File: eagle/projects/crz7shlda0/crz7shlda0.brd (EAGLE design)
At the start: 51.2 x 50 mm, 30 parts, among them J3 HDR-2X8, J5 HDR-2X8, Q1 BSS138, Q5 BSS138, Q6 BSS138, T1 MMBT3904

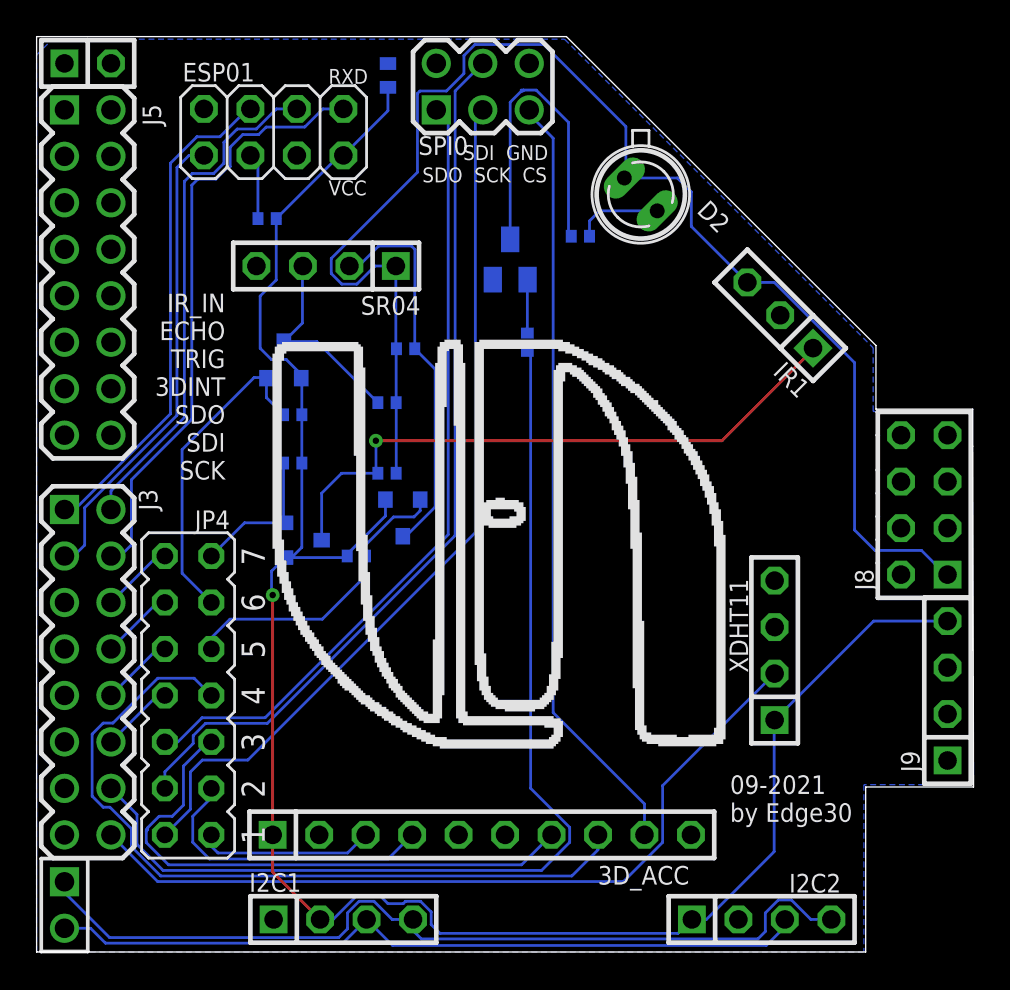
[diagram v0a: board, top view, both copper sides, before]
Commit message: cmod7shld0, crz7shlda0 production
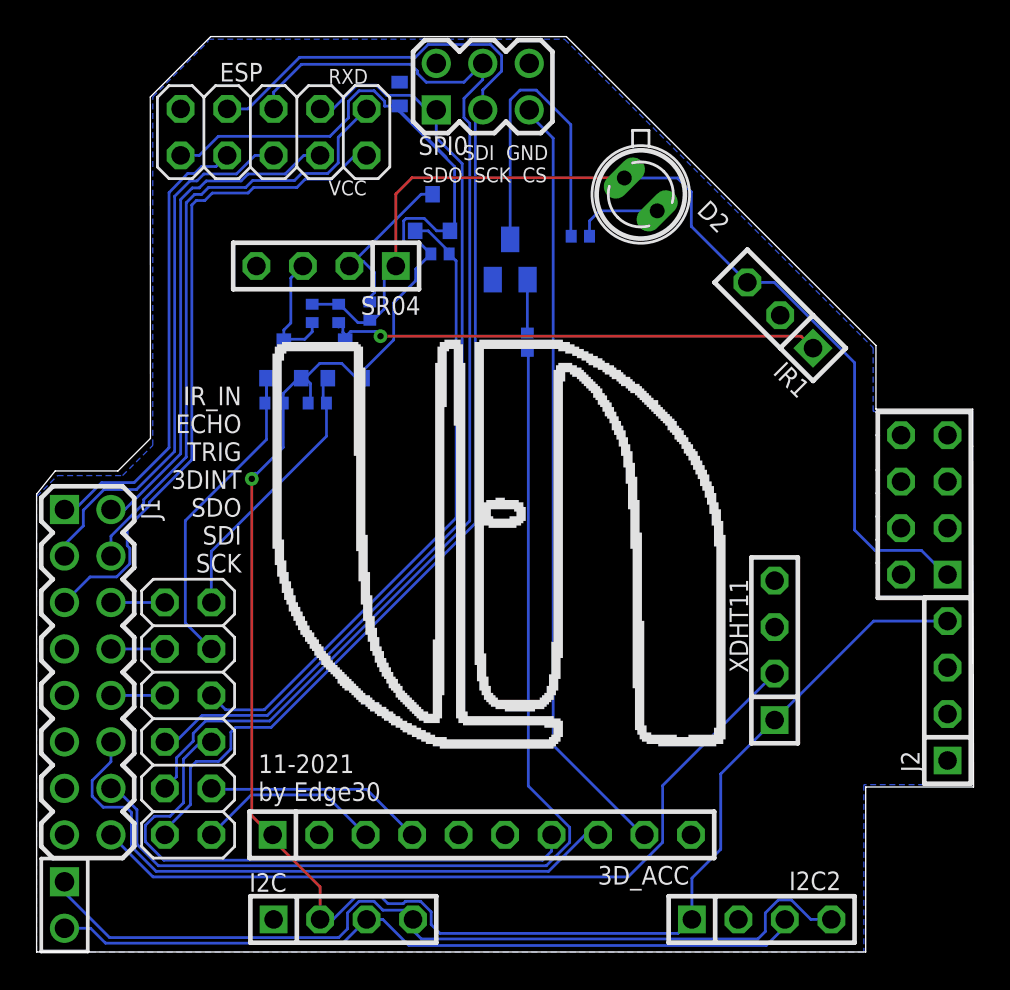
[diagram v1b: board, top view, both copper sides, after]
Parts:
- removed ESP01: (no value), pinhead:2X04
- removed J5: HDR-2X8, Mechanical:HDR-2X8
- removed J5G: (no value), pinhead2:1X02
- removed R19: 10k, rcl:R0402
- added ESP: (no value), pinhead:2X05
- I2C: value (none) -> I2C
- I2C2: value (none) -> I2Crev
- JP4: device jumper:JP7Q -> pinhead:2X06
- moved R17 17.1 mm to (22.0, 38.2)
- moved Q6 16.8 mm to (21.6, 40.4), turned to 0 degrees
- moved Q1 10.1 mm to (16.9, 32.4), turned to 0 degrees
- moved R14 9.13 mm to (16.5, 34.9), turned to 90 degrees
- moved R13 6.36 mm to (15.1, 34.9), turned to 90 degrees
- moved R15 3.54 mm to (15.3, 30.0), turned to 180 degrees
- moved R5 2.84 mm to (18.2, 35.0), turned to 270 degrees
- moved JP4 1.27 mm to (8.28, 12.8)
- moved C3 1.20 mm to (19.8, 46.9)
- moved R16 1.20 mm to (13.0, 30.0)
- renumbered I2C1 to I2C, J3 to J1, J9 to J2
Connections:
- removed net 3DIRQ: 3D_ACC.8, JP4.7
- removed net GPO0: ESP01.6, J1.2
- removed net GPO2: ESP01.4, J1.1
- removed net KCHIP_EN: ESP01.3, R19.2
- removed net URXD: ESP01.8, J1.4
- removed net UTXD: ESP01.1, J1.3
- new net CS2: ESP.10, J1.4
- new net EN_ESP: ESP.7, J1.2
- new net GPIO3: ESP.3, J1.1
- new net GPIO8: ESP.9, J1.5
- new net GPIO9: ESP.5, J1.3
- net 3D_INT: now also 3D_ACC.8; no longer JP4.8
- net ECHOIN: now also JP4.10; no longer JP4.12
- net ECHO_: now also JP4.9; no longer JP4.11
- net IRIN: now also JP4.12; no longer JP4.14
- net IR_OUT_: now also JP4.11; no longer JP4.13
- net K3V: now also ESP.1; no longer ESP01.7, R19.1
- net KGND: now also ESP.2; no longer ESP01.2, J5G.1, J5G.2
- net SCK: now also ESP.4
- net SDI: now also ESP.6
- net SDO: now also ESP.8
- net TRIGOUT: now also JP4.8; no longer JP4.10
- net TRIG_: now also JP4.7; no longer JP4.9
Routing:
- net 3DIRQ: track 43.0 -> 0.00 mm
- net GPIO8: track 0.00 -> 36.2 mm
- net CS2: track 0.00 -> 33.8 mm
- net URXD: track 33.0 -> 0.00 mm
- net 3D_INT: track 4.00 -> 34.7 mm
- net GPIO9: track 0.00 -> 29.5 mm
- net GPO0: track 28.1 -> 0.00 mm
- net EN_ESP: track 0.00 -> 27.6 mm
- net GPO2: track 27.3 -> 0.00 mm
- net UTXD: track 25.8 -> 0.00 mm
- net GPIO3: track 0.00 -> 25.1 mm
- net K5V: track 78.4 -> 57.4 mm
- net SCK: track 48.3 -> 68.8 mm
- net K3V: track 107.3 -> 126.8 mm
- net TRIG_: track 17.3 -> 35.4 mm
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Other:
- outline, holes or cut-outs redrawn
- board text added: "11-2021 by Edge30"
- board text removed: "09-2021 by Edge30"

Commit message: just push latest hanging changes to repo
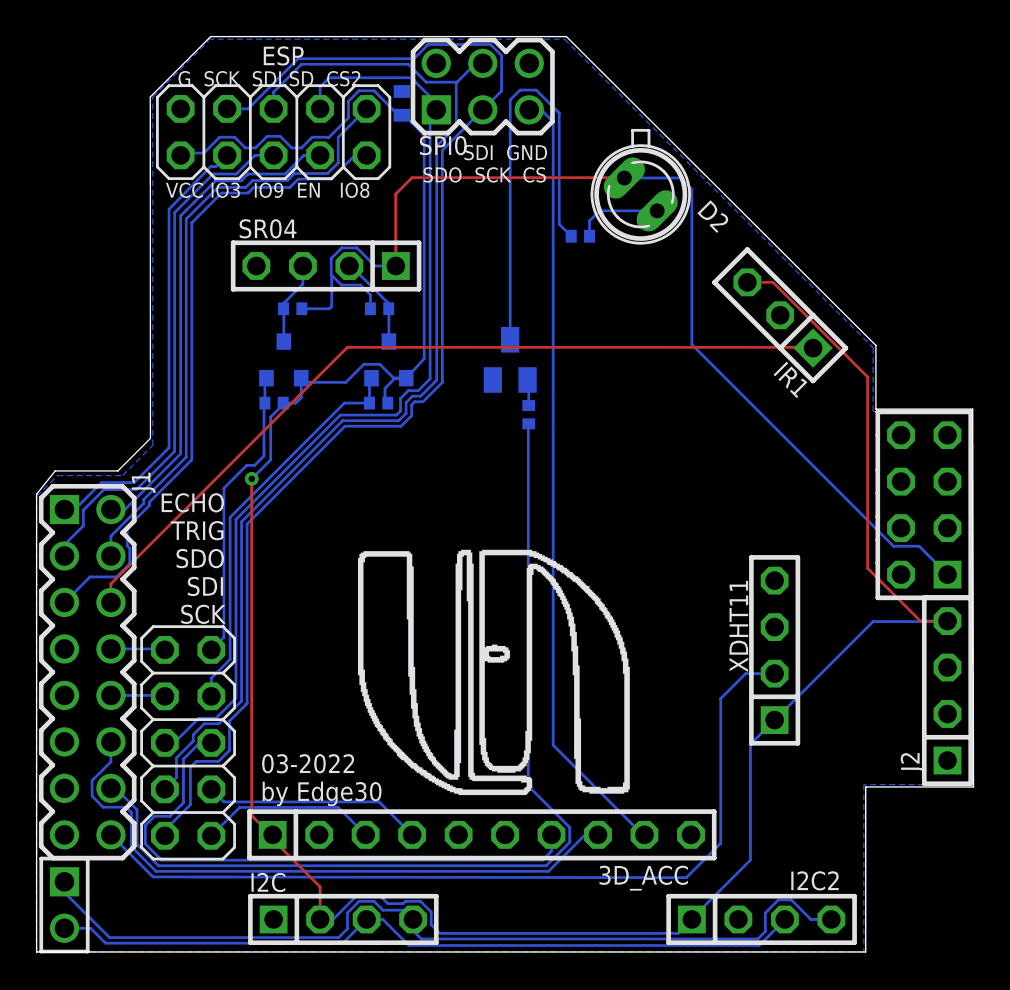
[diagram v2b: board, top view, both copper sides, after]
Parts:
- removed Q1: BSS138, bss138_10:SOT23
- removed R14, R15: 10k, rcl:R0402
- JP4: device pinhead:2X06 -> pinhead:2X05
- moved R17 8.82 mm to (18.7, 30.0), turned to 0 degrees
- moved Q6 8.40 mm to (19.3, 32.4)
- moved T1 5.49 mm to (25.9, 32.4)
- moved R18 3.96 mm to (26.9, 29.4)
- moved JP4 1.32 mm to (8.28, 11.4)
- moved R13 1.10 mm to (14.0, 35.2), turned to 180 degrees
- moved R5 0.55 mm to (18.7, 35.2), turned to 0 degrees
- moved C3 0.52 mm to (20.0, 46.4)
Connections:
- removed net IR_OUT: IR1.1, Q1.3, R14.1
- removed net IR_OUT_: JP4.11, Q1.2, R15.2
- net IRIN: now also IR1.1; no longer JP4.12
- net K3V: now also IR1.3; no longer Q1.1, R15.1
- net K5V: no longer IR1.3, R14.2
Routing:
- net IRIN: track 2.95 -> 44.8 mm
- net IR_OUT: track 28.0 -> 0.00 mm, vias 1 -> 0
- net K3V: track 126.8 -> 144.7 mm
- net IR_OUT_: track 15.0 -> 0.00 mm
- net TRIG_: track 35.4 -> 21.9 mm
- net N$3: track 18.0 -> 23.5 mm
- net TRIG: track 9.61 -> 5.08 mm
- net IROUT: track 56.3 -> 52.3 mm
- net SENSIN: track 43.6 -> 46.5 mm
- net K5V: track 57.4 -> 60.2 mm
- net ECHO: track 6.93 -> 4.58 mm
- net ECHO_: track 18.6 -> 16.3 mm
- net N$9: track 2.93 -> 1.47 mm
- net SDI: track 63.0 -> 61.6 mm
- net SCK: track 68.8 -> 70.2 mm
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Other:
- board text added: "03-2022 by Edge30"
- board text added: "ECHO TRIG SDO SDI SCK"
- board text added: "G SCK SDI SD CS2 VCC IO3 IO9 EN IO8"
- board text removed: "11-2021 by Edge30"
- board text removed: "IR_IN ECHO TRIG 3DINT SDO SDI SCK"
- board text removed: "RXD VCC"
